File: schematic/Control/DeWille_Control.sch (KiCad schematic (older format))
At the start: 8 parts, among them J101 HN2x10, J102 HN2x10, J103 HN2x10

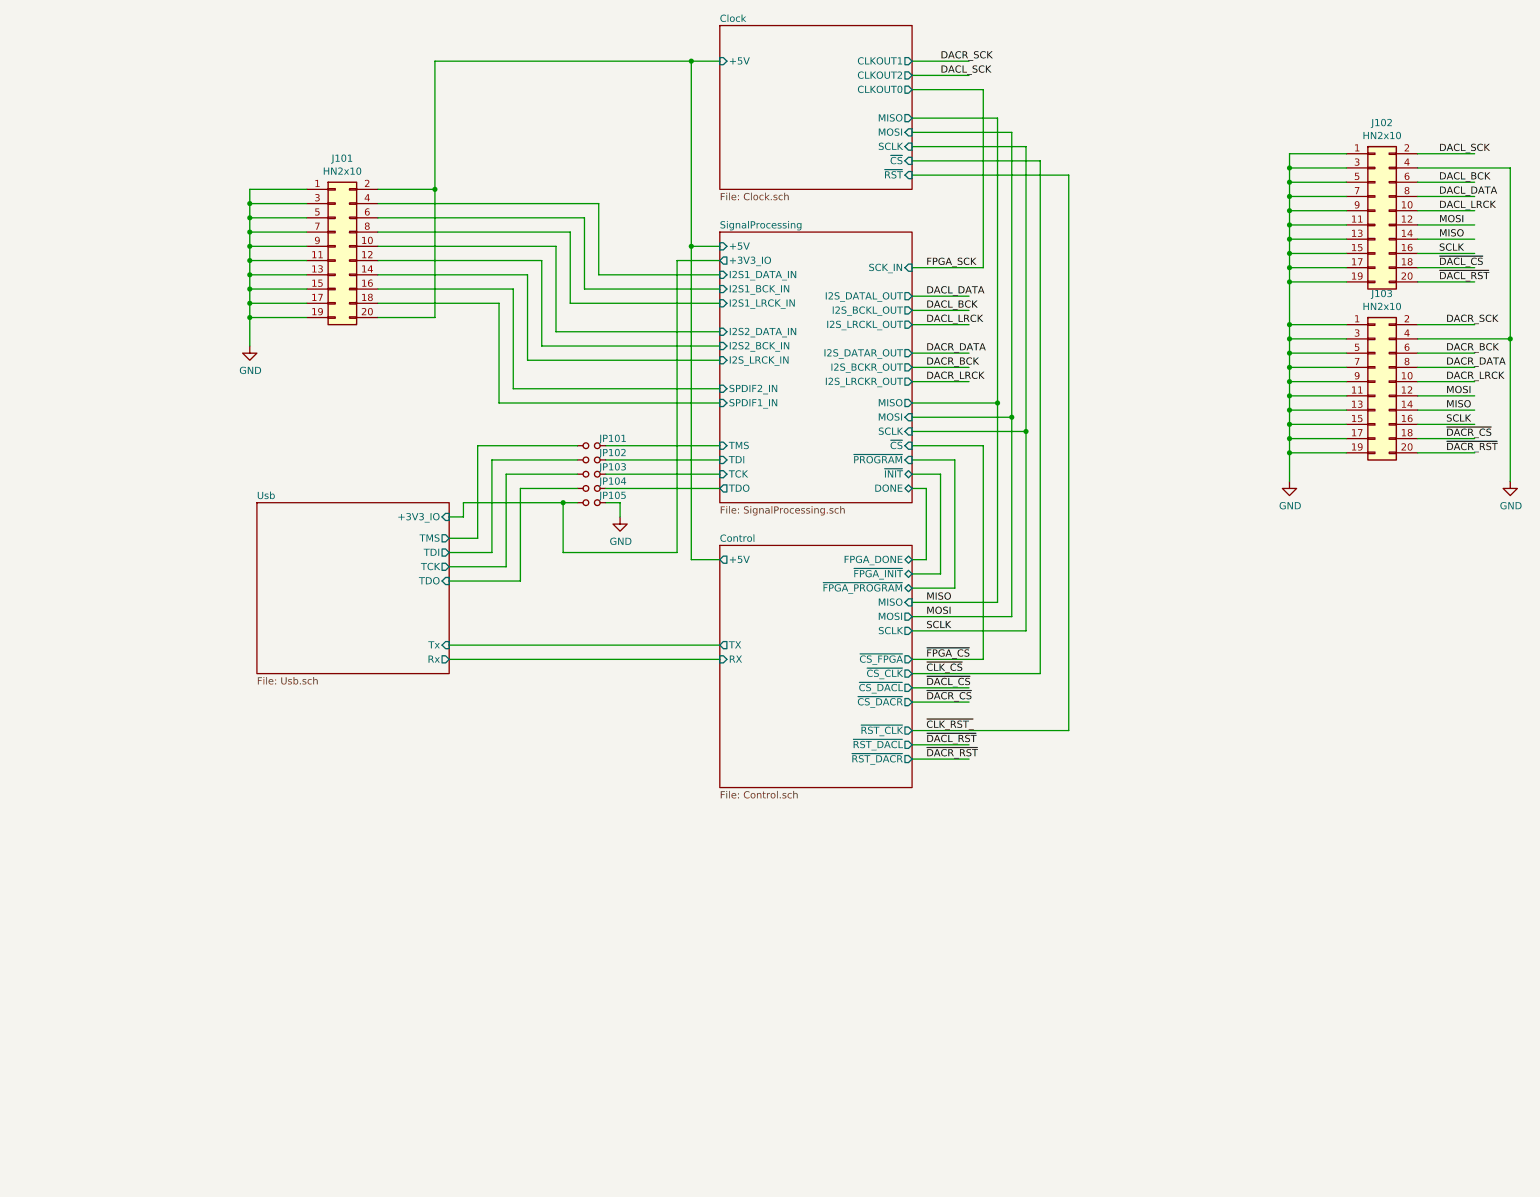
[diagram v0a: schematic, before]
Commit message: Interim commit
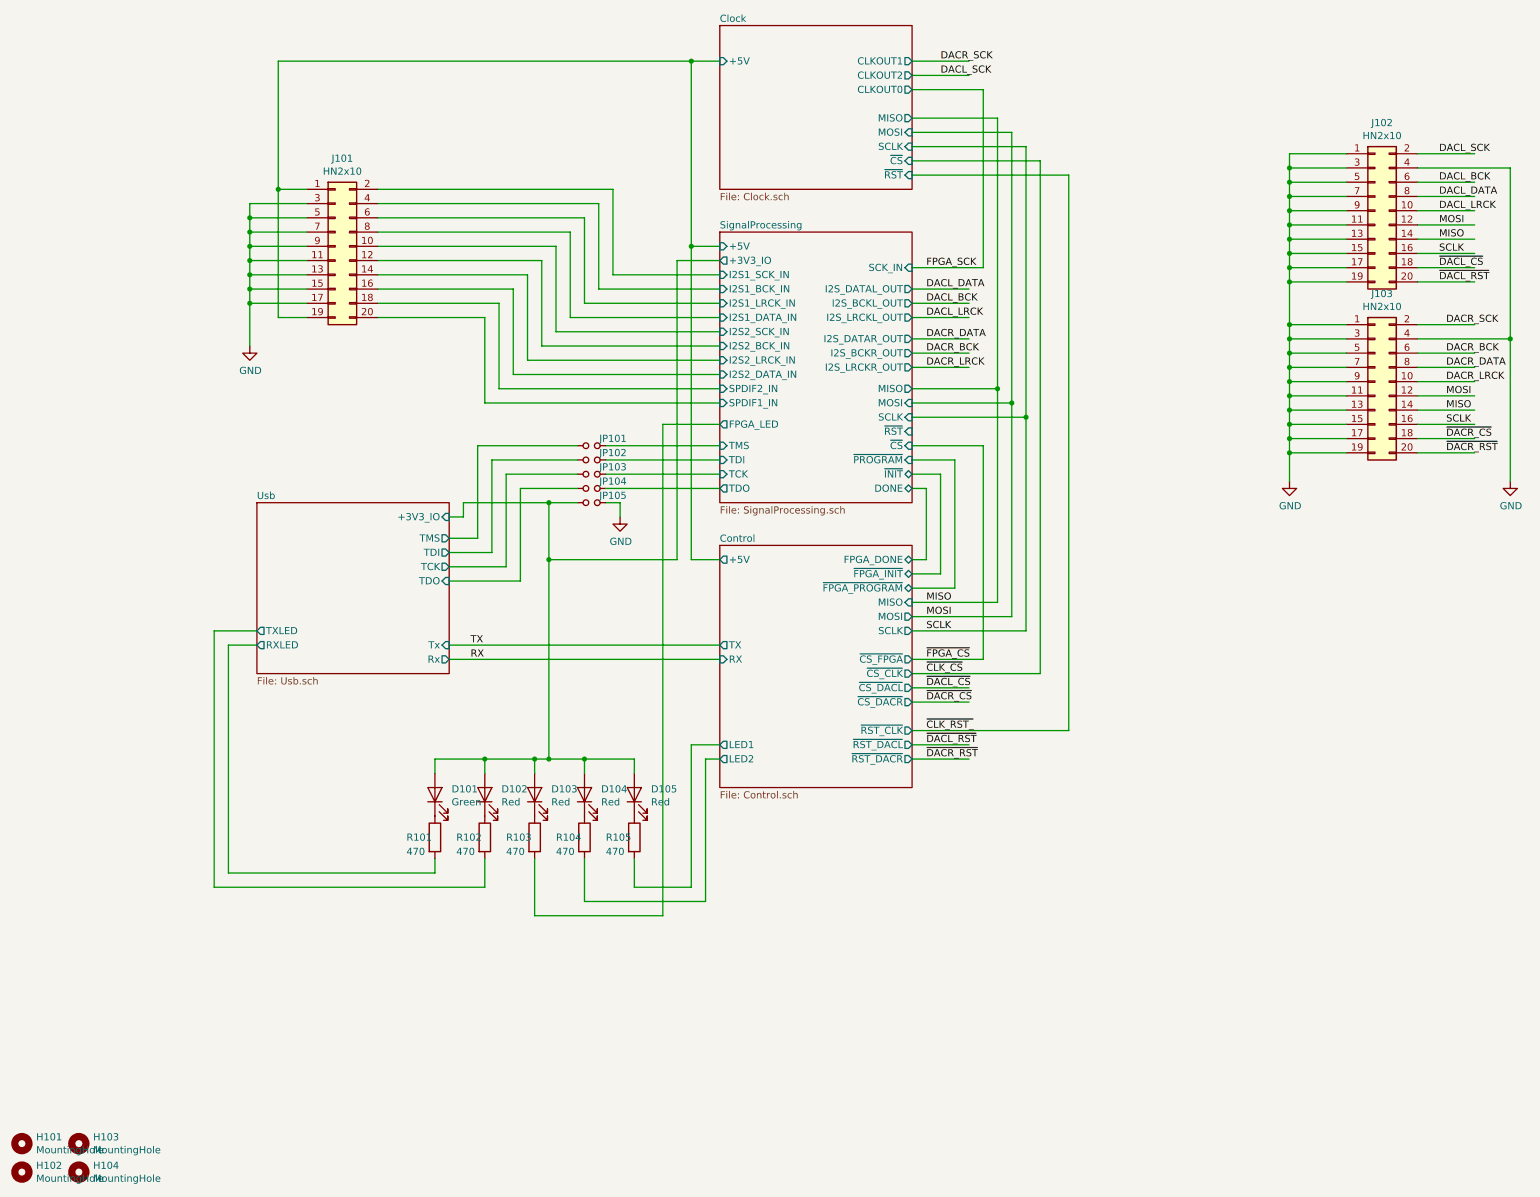
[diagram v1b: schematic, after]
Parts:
- added D101: Green, LED_SMD:LED_0805_2012Metric, symbol Device:LED
- added D102, D103, D104, D105: Red, LED_SMD:LED_0805_2012Metric, symbol Device:LED
- added H101, H102, H103, H104: MountingHole, MountingHole:MountingHole_3.2mm_M3_Pad, symbol Mechanical:MountingHole
- added R101, R102, R103, R104, R105: 470, Resistor_SMD:R_0603_1608Metric, symbol Device:R
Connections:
- net labels added: RX, TX
- wire segments 192 -> 225
